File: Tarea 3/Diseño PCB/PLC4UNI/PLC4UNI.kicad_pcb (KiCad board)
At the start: 4 copper layers, 100.1 x 80.2 mm, 137 parts, among them J1 Screw_Terminal_01x18, J2 Screw_Terminal_01x18, J4 Conn_01x03, K1 G5Q-1, K2 G5Q-1, Q1 BC108A, Q10 IRLML6402TRPBF-JSM, Q2 BC108A, Q3 BC108A, Q4 TIP41, Q5 IRLML0040, Q6 TIP41, Q7 IRLML0040, Q8 BC108A, Q9 IRLML0040, U1 ESP32-S3-WROOM-1, U18 TLP290, U2 AP63203WU, U3 GP8303-TC50-EW, U4 TLP290

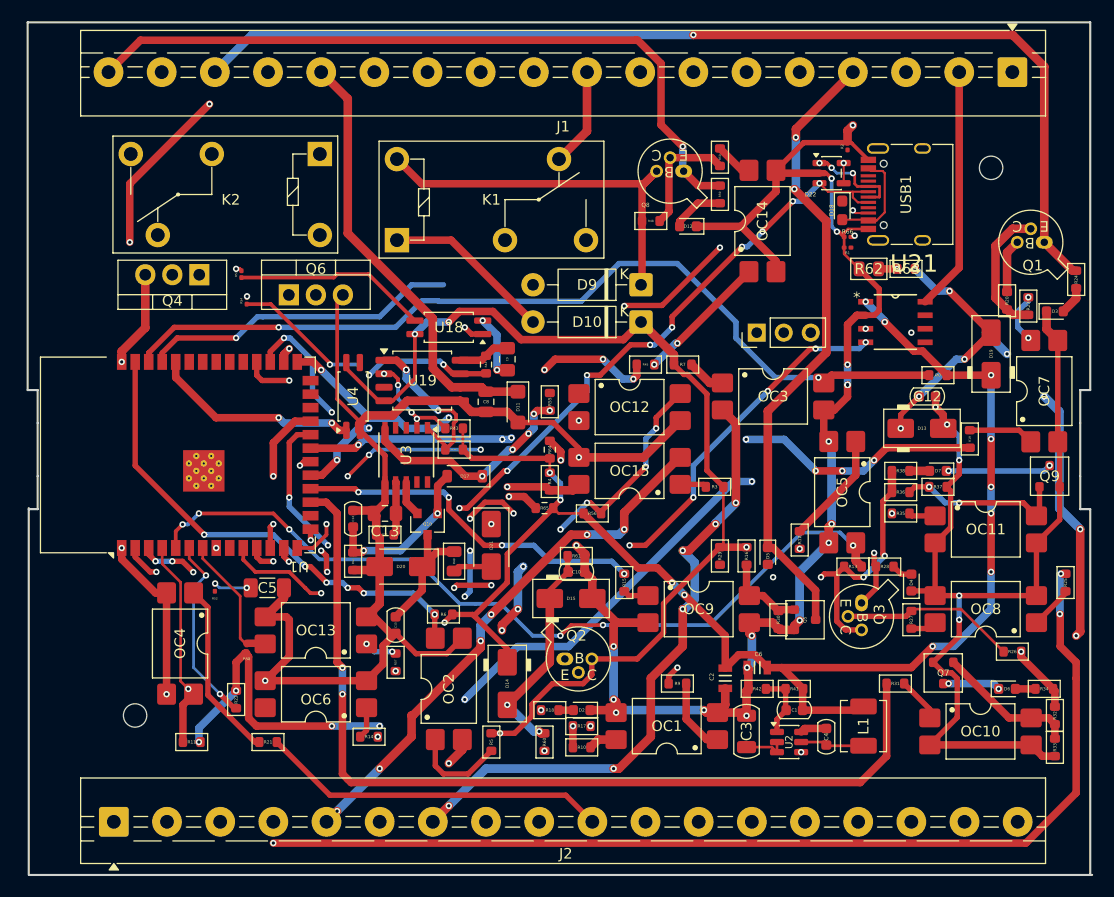
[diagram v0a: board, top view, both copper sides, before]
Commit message: Tarea - Update
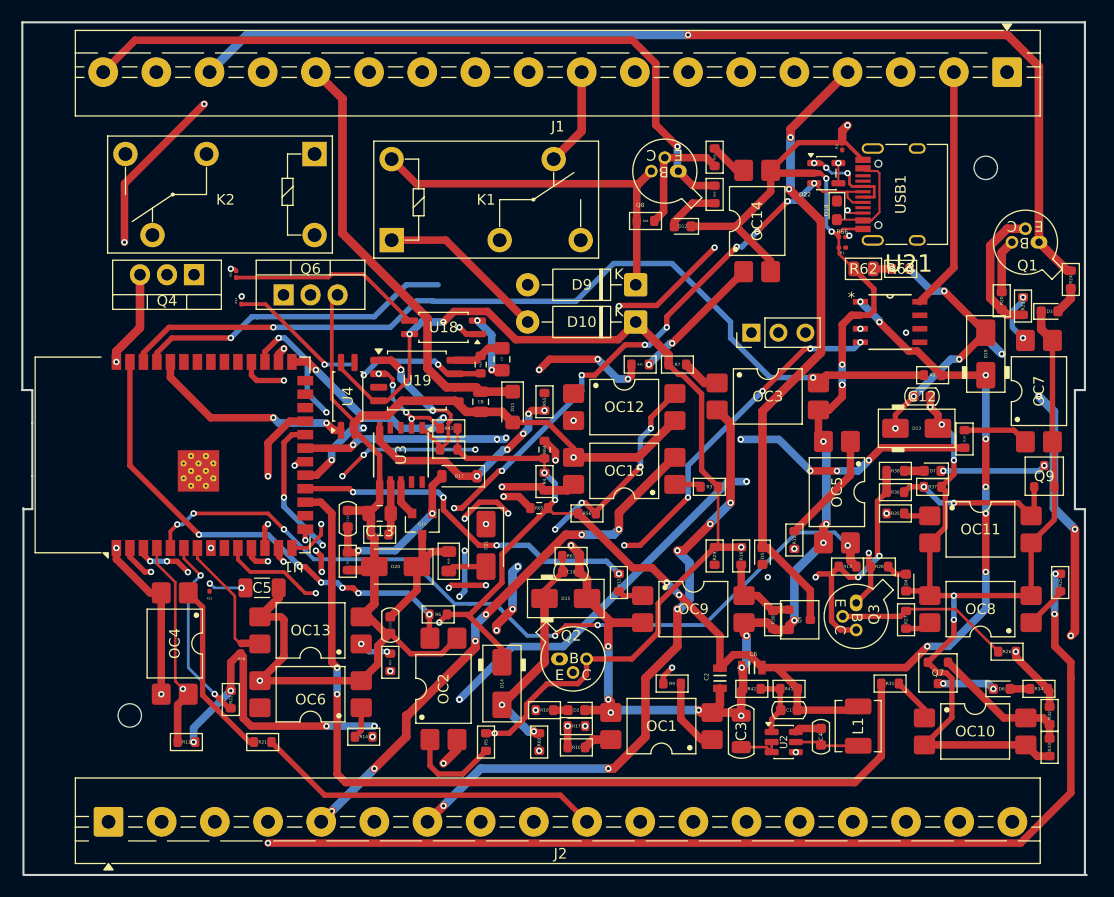
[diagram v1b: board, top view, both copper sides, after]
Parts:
- moved C1 0.50 mm to (134.5, 100.0)
- moved C10 0.50 mm to (114.0, 87.0)
- moved C12 0.50 mm to (147.0, 70.5)
- moved C13 0.50 mm to (96.0, 81.5)
- moved C14 0.50 mm to (93.0, 82.0)
- moved C15 0.50 mm to (97.0, 92.0)
- moved C2 0.50 mm to (128.0, 97.0)
- moved C3 0.50 mm to (130.0, 102.0)
- moved C4 0.50 mm to (137.5, 102.5)
- moved C5 0.50 mm to (84.9, 88.5)
- moved C6 0.50 mm to (131.0, 96.0)
- moved C8 0.50 mm to (105.5, 71.0)
- moved C9 0.50 mm to (107.5, 67.0)
- moved D10 0.50 mm to (120.1, 63.5)
- moved D11 0.50 mm to (108.5, 71.5)
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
